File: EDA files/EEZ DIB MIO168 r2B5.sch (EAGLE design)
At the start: 254 parts, among them IC1 M24C32-WMN6P, IC10 OPA2196IDR, IC11 DAC7760IPWPR, IC12 DAC7760IPWPR, IC13 OPA376AIDBVR, IC14 DAC7563TDGSR, IC15 OPA2196IDR, IC16 BTS3408G, IC17 BTS3408G, IC18 BTS3408G, IC19 BTS3408G, IC2 Si8641BB-B-IS1, IC20 TL431B, IC21 DG212BDY-T1-E3, IC22 74HC126PW,118, IC3 Si8641BB-B-IS1, IC4 LP2985-33DBVR, IC5 L78L15, IC6 SN6505BDBVT, IC7 L79L15, IC8 STM32F446ZCT6, IC9 N.C., J1 4907, J2 N.C., Q1 2N7002PS,115, Q10 MMBT5551, Q11 2N7002, Q2 2N7002PS,115, Q3 2N7002PS,115, Q4 2N7002PS,115, Q5 2N7002PS,115, Q6 BSS84P, Q7 MMBT5401, Q8 BSS84P, Q9 MMBT5551, X1 77317-104-28LF, X2 N.C., X3 691327310016, X4 691322310008, X5 DS1014-10RF1B, X6 DS1014-10RF1B, X7 DS1023-2*14S21, X8 DS1023-2*14S21, Y1 LF XTAL026392

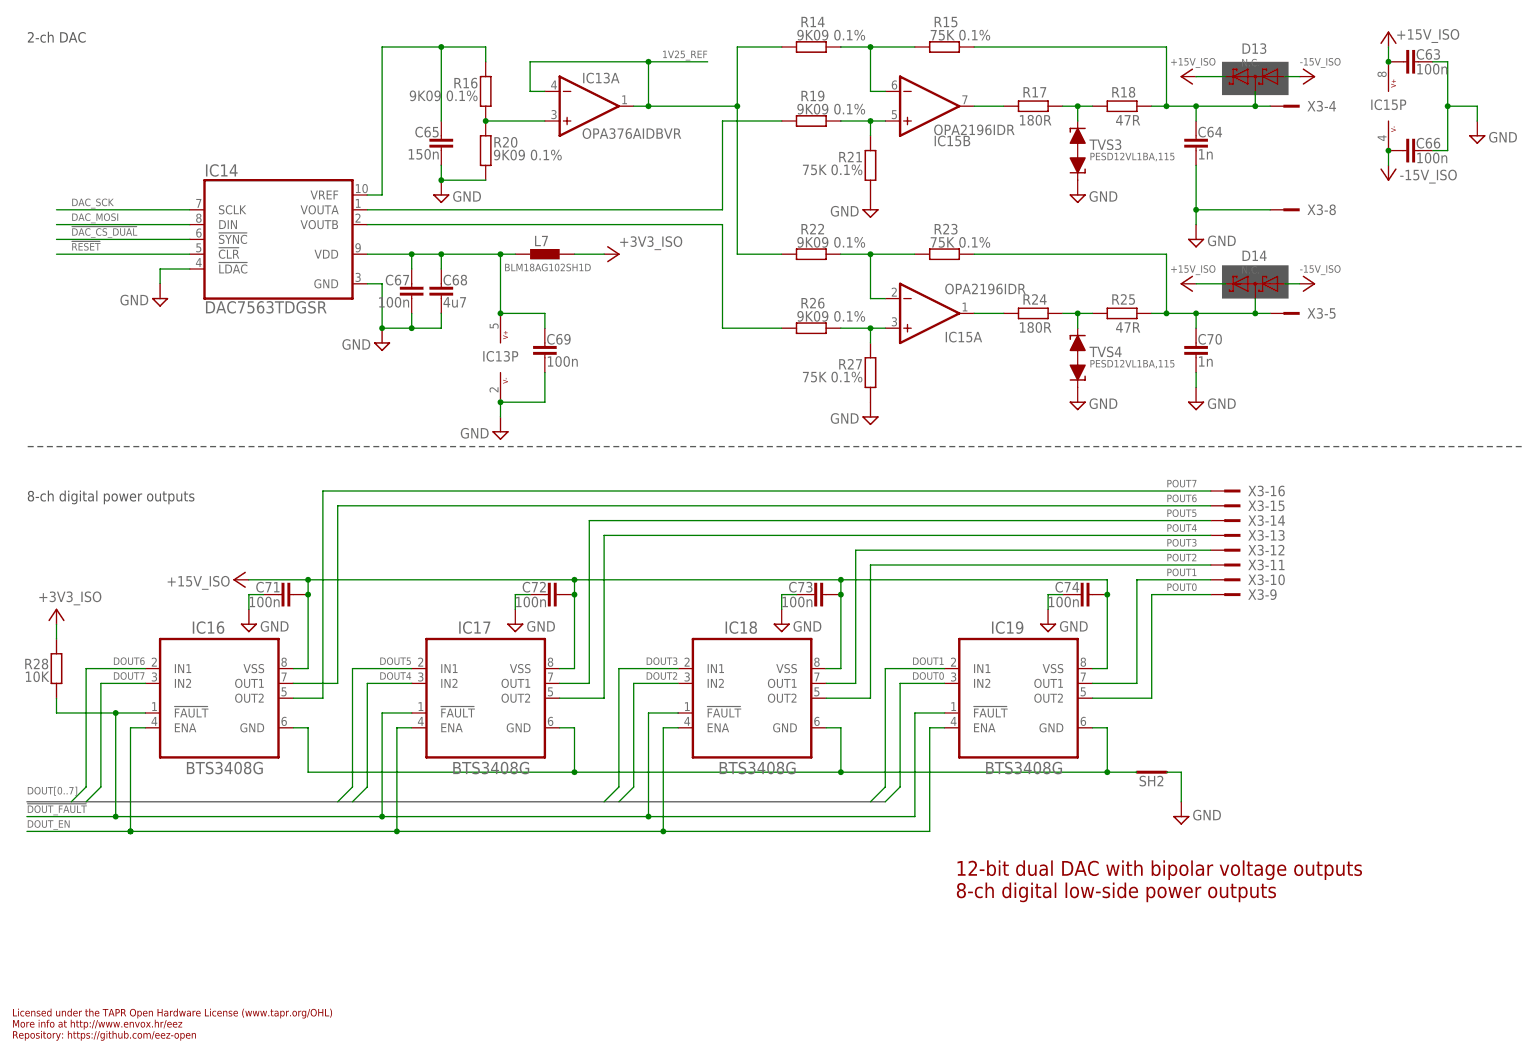
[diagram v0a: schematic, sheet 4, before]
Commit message: BOM update
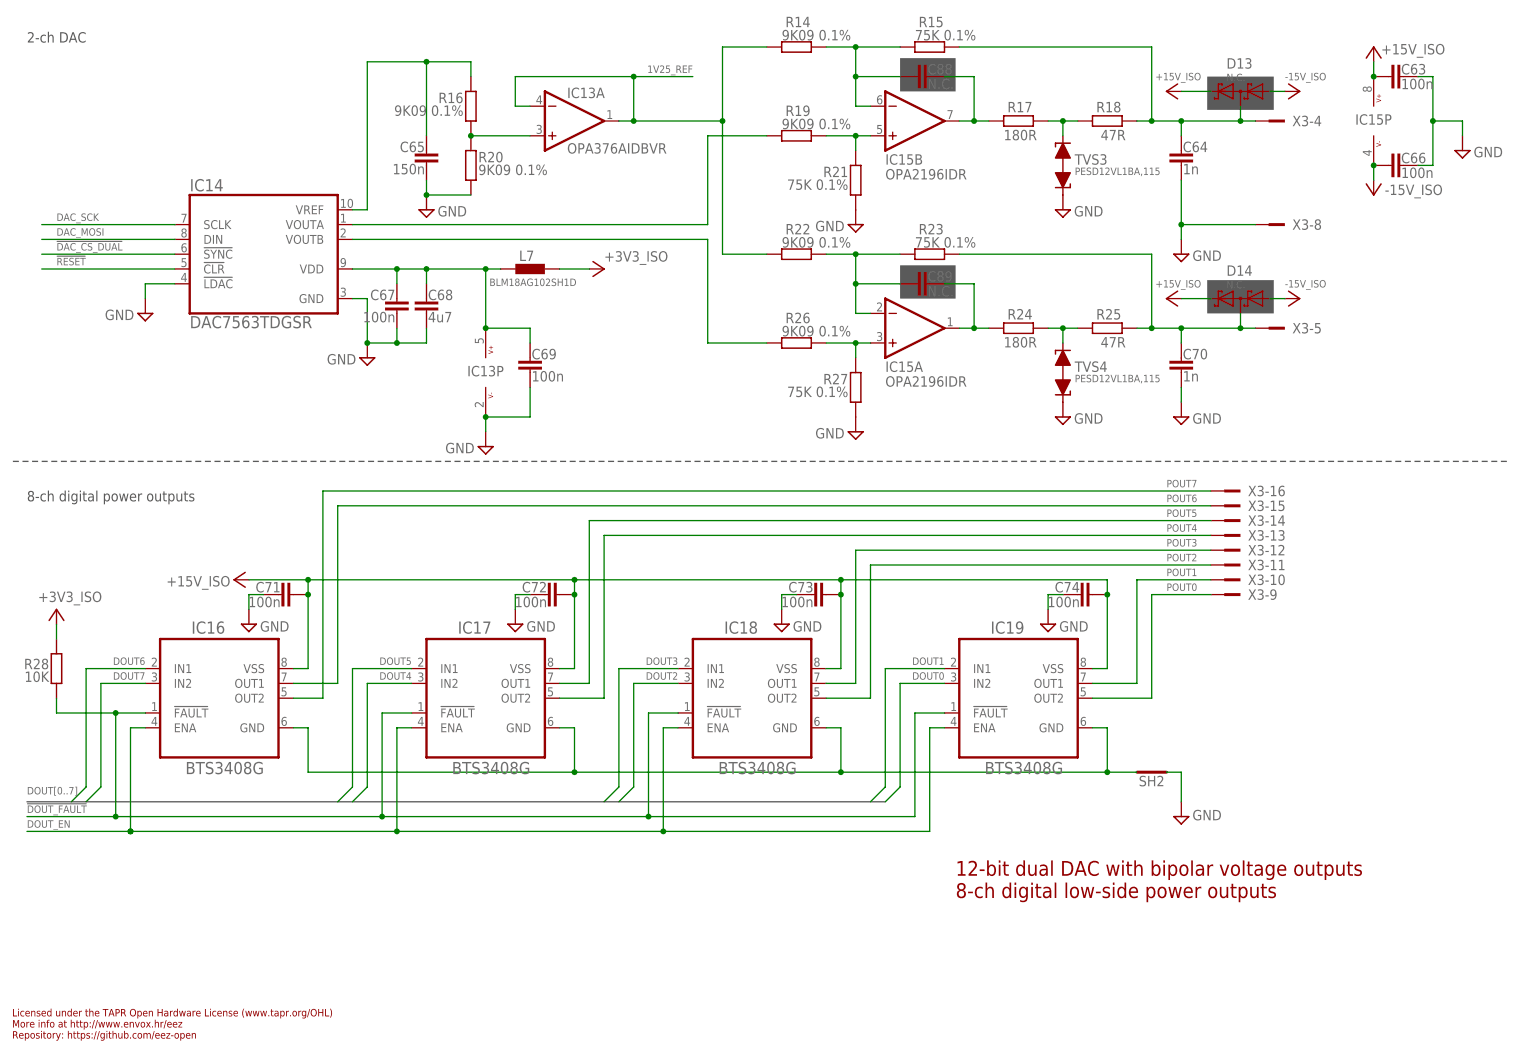
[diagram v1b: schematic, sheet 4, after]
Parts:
- added C88, C89: N.C., rcl:C-EUC0805
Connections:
- net N$55: now also C88.1
- net N$56: now also C88.2
- net N$58: now also C89.1
- net N$59: now also C89.2
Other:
- moved on the sheet: C63, C64, C65, C66, C67, C68, C69, C70, D13, D14, IC13A, IC13P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
